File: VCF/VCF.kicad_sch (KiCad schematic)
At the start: 64 parts, among them J1 AUDIO_IN, J2 CV1, J3 CV2, J4 AUDIO_OUT, J5 Conn_02x05_Odd_Even, J6 Conn_01x05_Male, J7 Conn_01x05_Female, J8 Conn_01x08_Male, J9 Conn_01x08_Female, SW1 SW_DPDT_x2, U1 TL074, U2 TL074

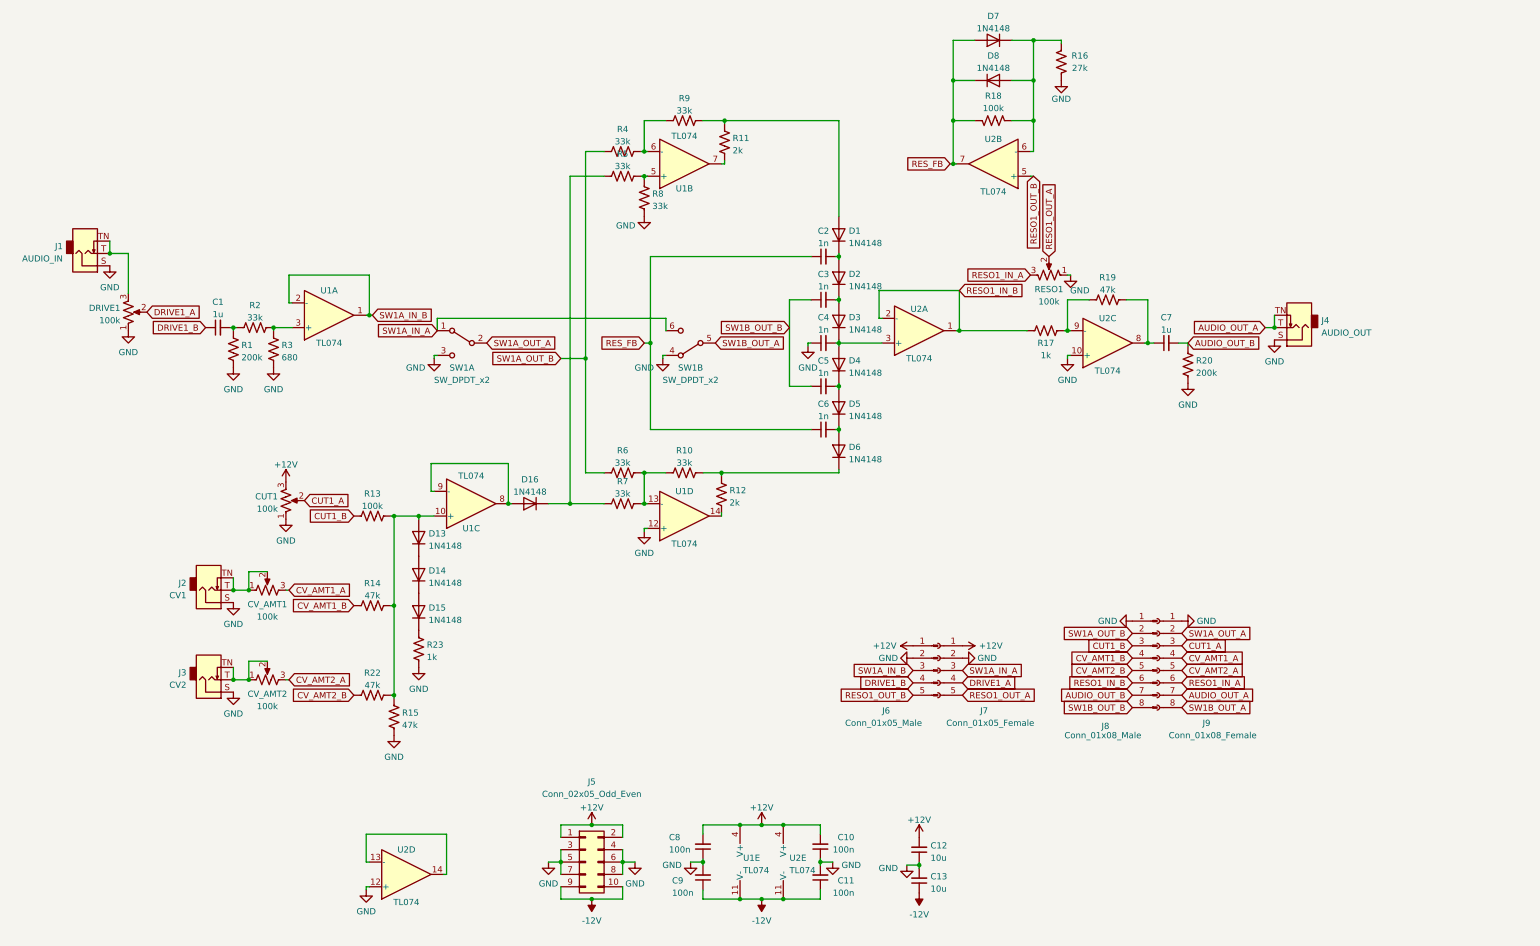
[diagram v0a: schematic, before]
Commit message: Updated PCBs
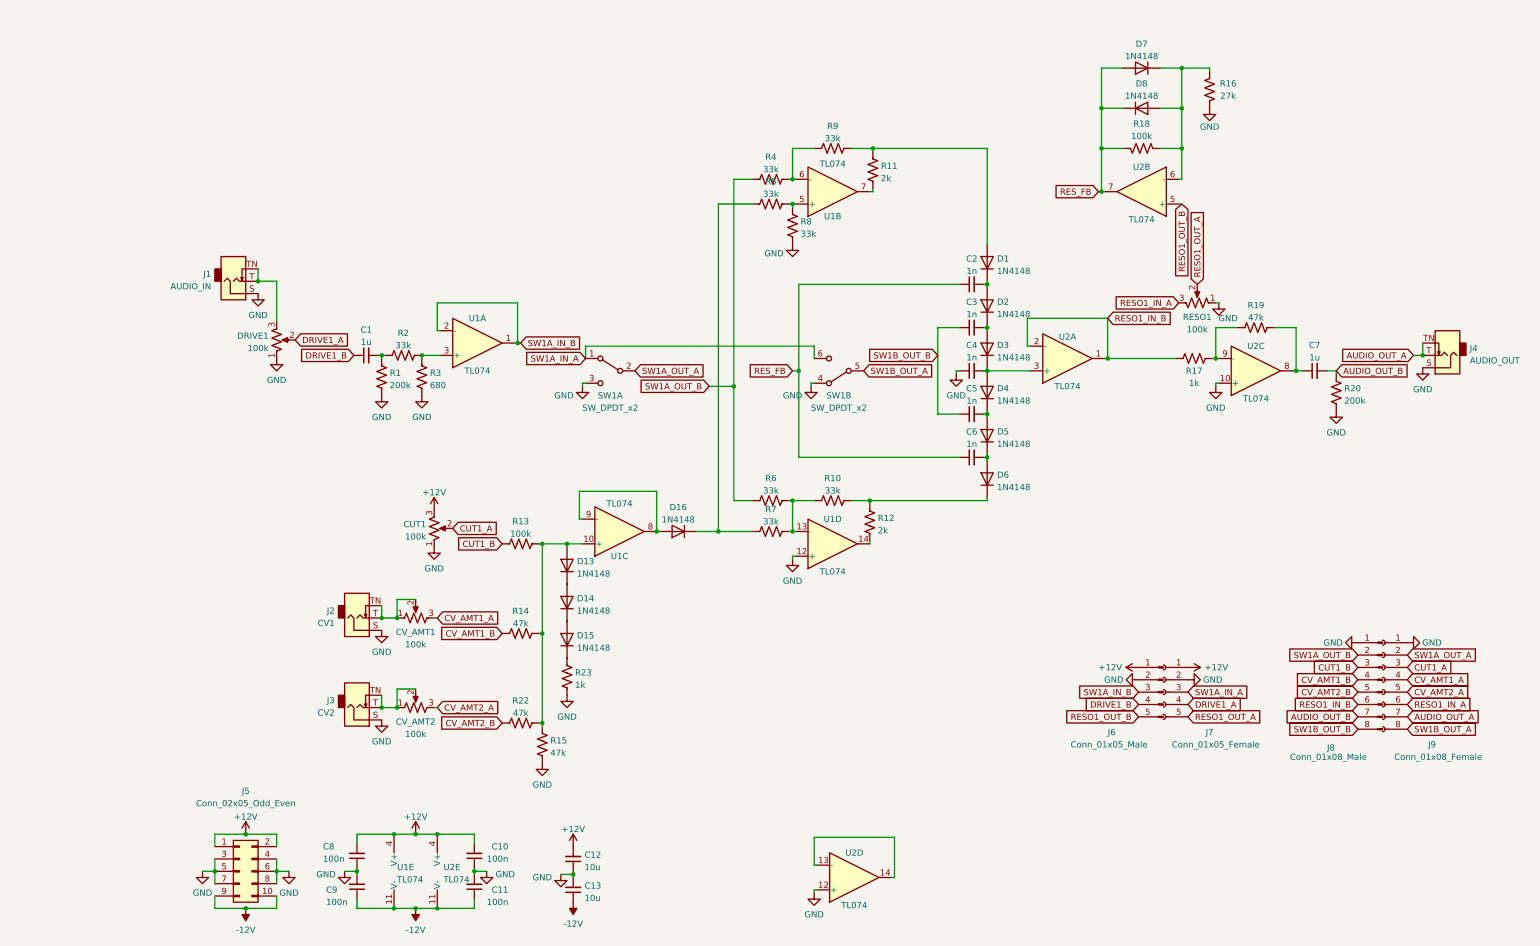
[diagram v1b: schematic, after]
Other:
- company: (none) -> Drachma Mfg
- title: (none) -> Moritz Klein Diode Ladder VCF
- moved on the sheet: C1, C10, C11, C12, C13, C2, C3, C4, C5, C6, C7, C8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
